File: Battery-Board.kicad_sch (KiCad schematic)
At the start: 20 parts, among them J6 Female Conn, J7 BATT IN, U17 AZ1084-3.3, U4 AZ1084-5.0

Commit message: A
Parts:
- R43, R44, R45: footprint Resistor_SMD:R_0603_1608Metric -> Resistor_SMD:R_0805_2012Metric
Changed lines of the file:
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@@
 	(label "OUT_{12V}"
 		(at 111.76 96.52 0)
+		(fields_autoplaced yes)
 		(effects
 			(font
@@
 	(label "CANL"
 		(at 165.1 109.22 270)
+		(fields_autoplaced yes)
 		(effects
 			(font
@@
 	(label "IN_{24V}"
 		(at 57.15 83.82 180)
+		(fields_autoplaced yes)
 		(effects
 			(font
@@
 	(label "CANH"
 		(at 162.56 109.22 270)
+		(fields_autoplaced yes)
 		(effects
 			(font
@@
 	(label "OUT_{7V}"
 		(at 111.76 81.28 0)
+		(fields_autoplaced yes)
 		(effects
 			(font
@@
 			)
 		)
-		(property "Footprint" "Resistor_SMD:R_0603_1608Metric"
+		(property "Footprint" "Resistor_SMD:R_0805_2012Metric"
 			(at 155.702 163.83 90)
 			(effects
@@
 			)
 		)
-		(property "Footprint" "Resistor_SMD:R_0603_1608Metric"
+		(property "Footprint" "Resistor_SMD:R_0805_2012Metric"
 			(at 89.662 163.83 90)
 			(effects
@@
 			)
 		)
-		(property "Footprint" "Resistor_SMD:R_0603_1608Metric"
+		(property "Footprint" "Resistor_SMD:R_0805_2012Metric"
 			(at 49.022 95.25 90)
 			(effects

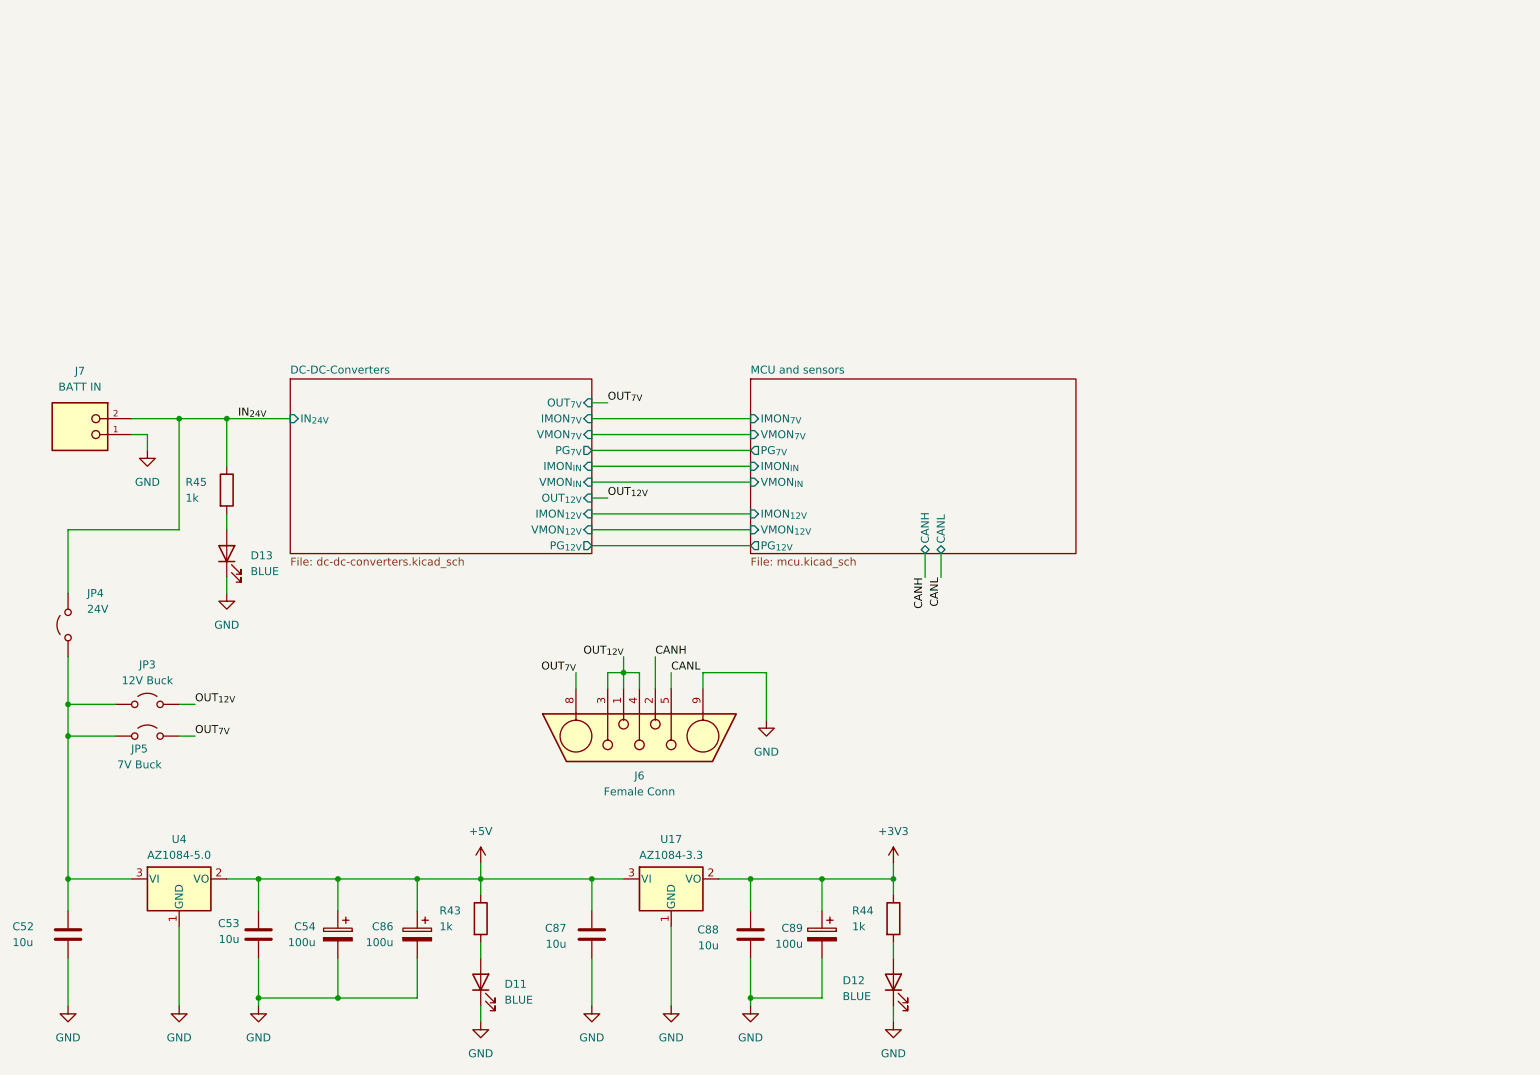
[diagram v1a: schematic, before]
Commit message: Done
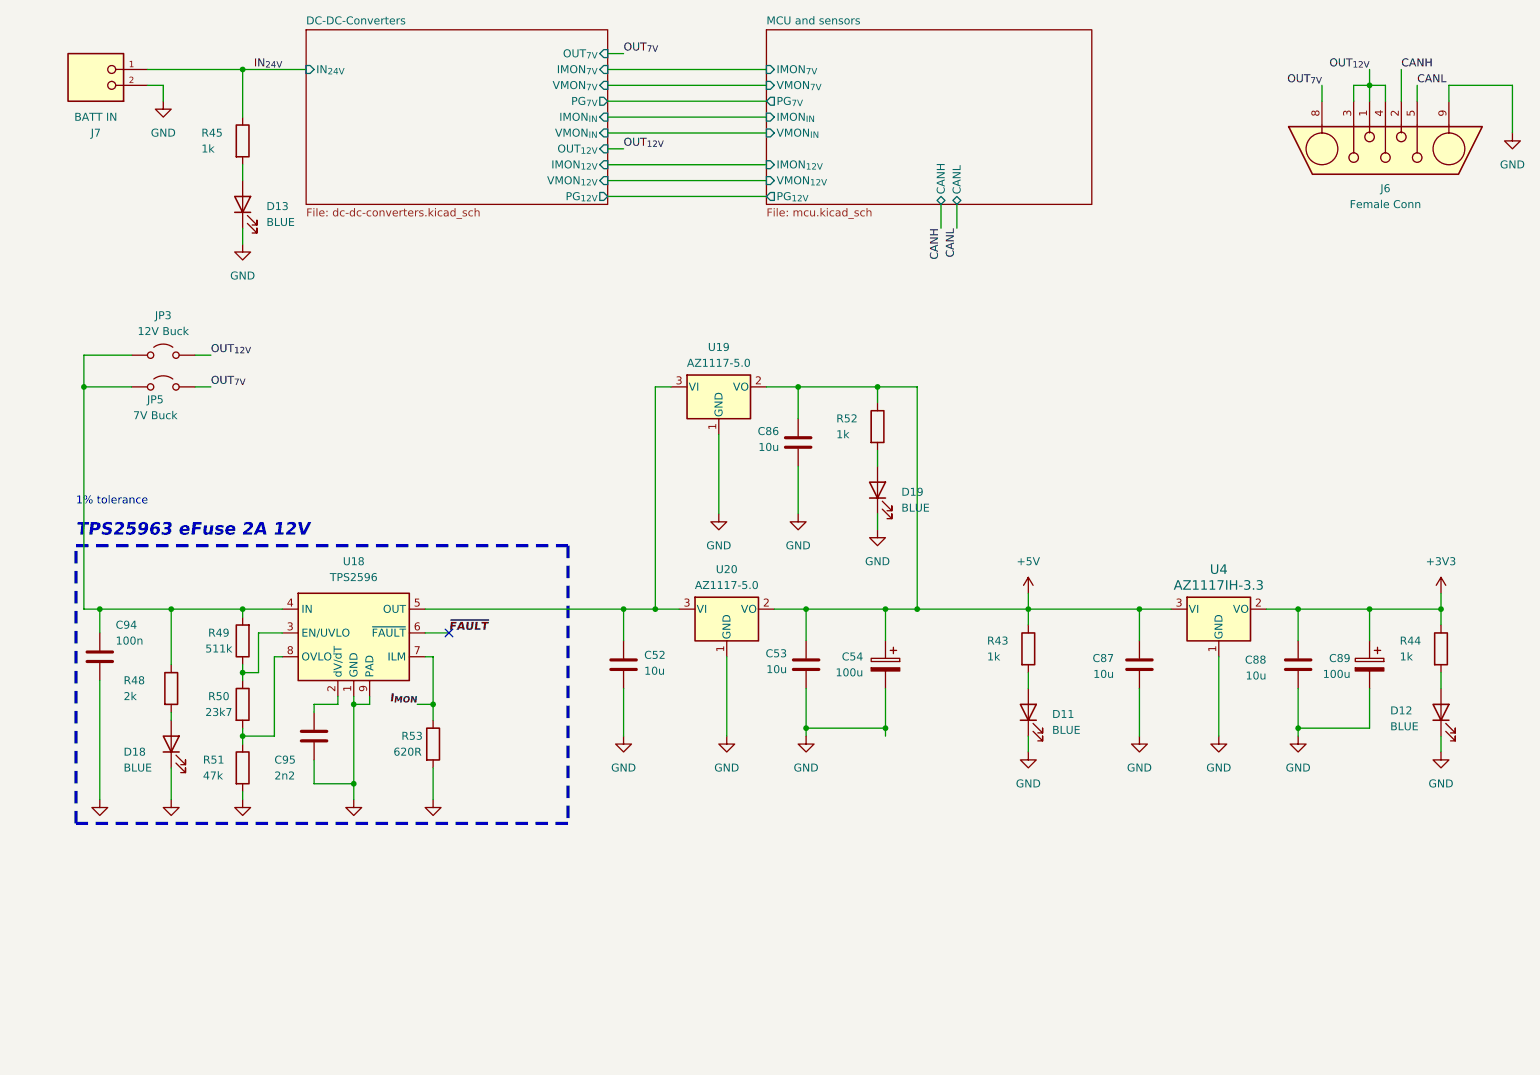
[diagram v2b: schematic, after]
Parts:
- removed C86: 100u, Capacitor_SMD:CP_Elec_6.3x9.9, symbol Device:C_Polarized
- removed JP4: 24V, symbol Jumper:Jumper_2_Open
- removed U17: AZ1084-3.3, Package_TO_SOT_SMD:TO-252-2, symbol Regulator_Linear:AZ1084-3.3
- removed U4: AZ1084-5.0, Package_TO_SOT_SMD:TO-252-2, symbol Regulator_Linear:AZ1084-5.0
- added C86: 10u, Capacitor_SMD:C_0805_2012Metric, symbol Device:C
- added C94: 100n, Capacitor_SMD:C_0603_1608Metric, symbol Device:C
- added C95: 2n2, Capacitor_SMD:C_0603_1608Metric, symbol Device:C
- added D18, D19: BLUE, LED_SMD:LED_0603_1608Metric, symbol Device:LED
- added R48: 2k, Resistor_SMD:R_0603_1608Metric, symbol Device:R
- added R49: 511k, Resistor_SMD:R_0603_1608Metric, symbol Device:R
- added R50: 23k7, Resistor_SMD:R_0603_1608Metric, symbol Device:R
- added R51: 47k, Resistor_SMD:R_0603_1608Metric, symbol Device:R
- added R52: 1k, Resistor_SMD:R_0603_1608Metric, symbol Device:R
- added R53: 620R, Resistor_SMD:R_0603_1608Metric, symbol Device:R
- added U18: TPS2596, Package_SO:TI_SO-PowerPAD-8, symbol H2_Parts:TPS2596
- added U19, U20: AZ1117-5.0, Package_TO_SOT_SMD:SOT-223-3_TabPin2, symbol Regulator_Linear:AZ1117-5.0
- added U4: AZ1117IH-3.3, Package_TO_SOT_SMD:SOT-223-3_TabPin2, symbol ecocad_lib_symbols:AZ1117IH-3.3
- JP3, JP5: footprint (none) -> ecocad_lib_footprints:J_0603_Triangular
- R43, R44, R45: footprint Resistor_SMD:R_0805_2012Metric -> Resistor_SMD:R_0603_1608Metric
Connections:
- net +3V3: now also U4.2 (VO)
- net +5V: now also C86.1, R52.1, U19.2 (VO), U20.2 (VO), U4.3 (VI)
- net GND: now also J7.2, C86.2, C94.2, C95.2, D18.1 (K), D19.1 (K), R51.2, R53.2, U18.1 (GND), U18.9 (PAD), U19.1 (GND), U20.1 (GND), U4.1 (GND); no longer J7.1
- net IN_{24V}: now also J7.1; no longer J7.2
- net at JP3.1 (A), JP5.1 (A): now also C94.1, R48.1, R49.2, U18.4 (IN); no longer C52.1
- new net: C52.1, U18.5 (OUT), U19.3 (VI), U20.3 (VI)
- new net: D19.2 (A), R52.2
- new net: R49.1, R50.1, U18.3 (EN/UVLO)
- new net: C95.1, U18.2 (dV/dT)
- new net: R50.2, R51.1, U18.8 (OVLO)
- new net: D18.2 (A), R48.2
- new net I_{MON}: R53.1, U18.7 (ILM)
- new net ~{FAULT}: U18.6 (~{FAULT})
- no-connect marks 0 -> 1
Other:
- note added: "1% tolerance"
- note added: "TPS25963 eFuse 2A 12V"
- moved on the sheet: C52, C53, C54, C87, C88, C89, D11, D12, D13, J6, J7, JP3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
